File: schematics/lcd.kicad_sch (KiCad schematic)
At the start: 4 parts, among them U27 ATF22V10C-7, U28 74HC373

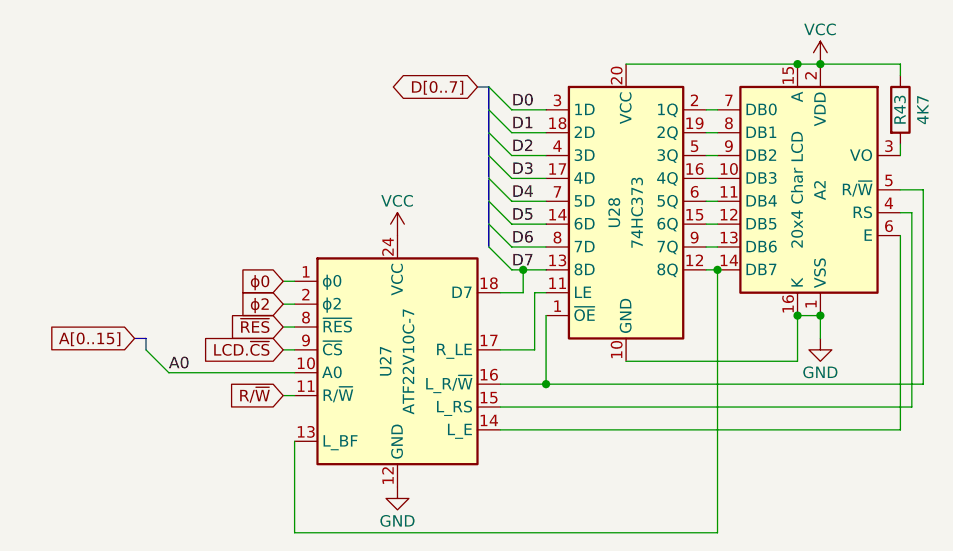
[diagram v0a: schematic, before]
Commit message: clock improvements
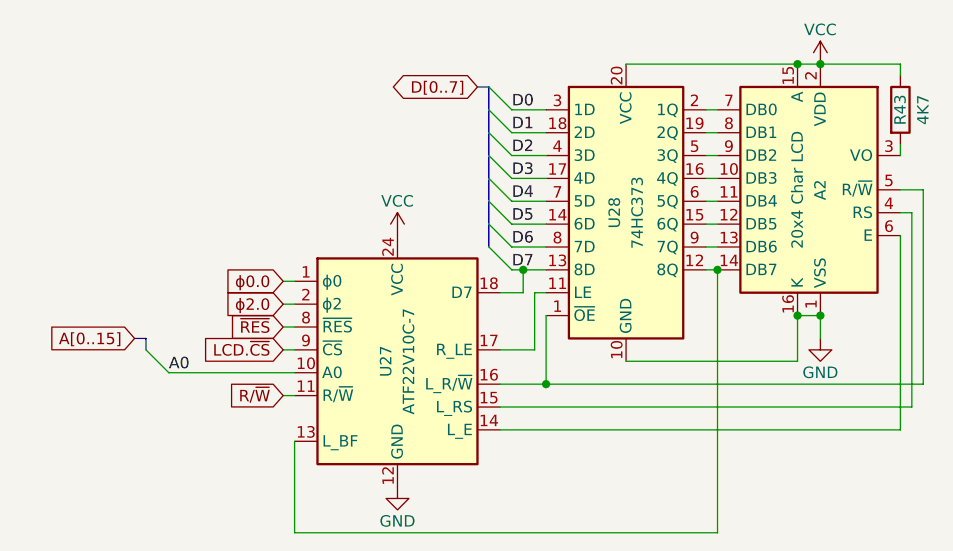
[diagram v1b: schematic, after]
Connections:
- net ϕ0 renamed ϕ0.0
- net ϕ2 renamed ϕ2.0
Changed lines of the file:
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@@
 		)
 	)
-	(global_label "ϕ0"
+	(global_label "ϕ0.0"
 		(shape input)
 		(at 104.14 99.06 180)
@@
 		)
 		(property "Intersheetrefs" "${INTERSHEET_REFS}"
-			(at 98.6148 99.06 0)
+			(at 96.8005 99.06 0)
 			(hide yes)
 			(show_name no)
@@
 		)
 	)
-	(global_label "ϕ2"
+	(global_label "ϕ2.0"
 		(shape input)
 		(at 104.14 101.6 180)
@@
 		)
 		(property "Intersheetrefs" "${INTERSHEET_REFS}"
-			(at 98.6148 101.6 0)
+			(at 96.8005 101.6 0)
 			(hide yes)
 			(show_name no)
